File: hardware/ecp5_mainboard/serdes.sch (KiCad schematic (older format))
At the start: 48 parts, among them J14 9774025151R, J8 9774025151R, P1 M2_SOCKET_E, P3 PCIe_x4_EDGE, U11 CBTL02043A, U15 ECP5UM5G_85_CABGA756, U16 5P49V6965, Y1 25MHz

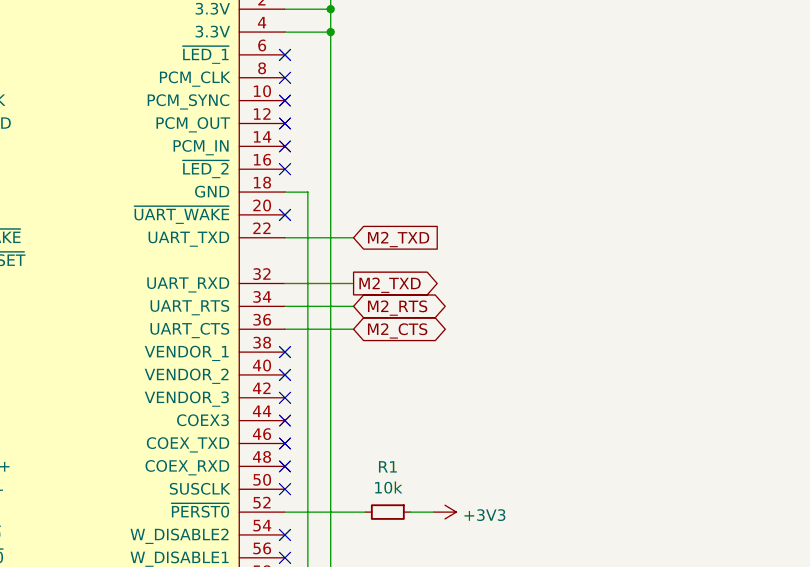
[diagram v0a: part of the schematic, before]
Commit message: hardware/mainboard: Clock & M.2 routing
Signed-off-by: David Shah <davey1576@gmail.com>
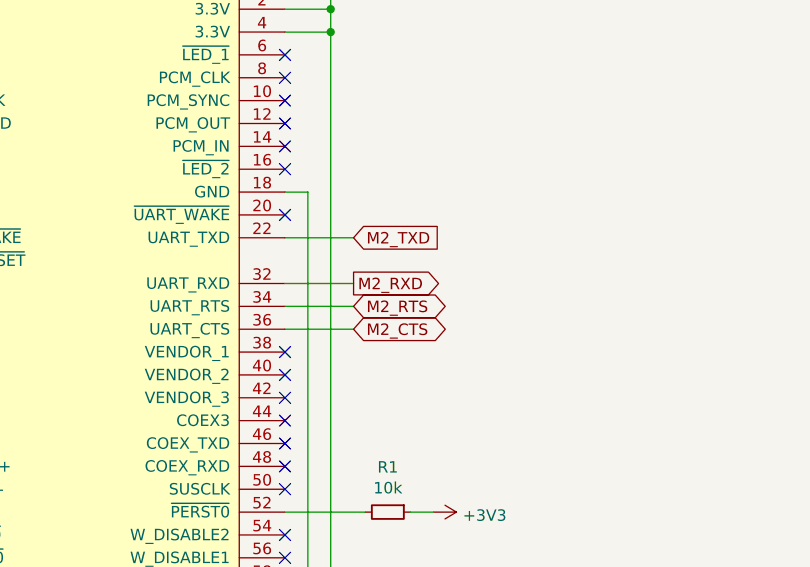
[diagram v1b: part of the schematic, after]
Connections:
- net M2_TXD: no longer P1.32 (UART_RXD)
- new net M2_RXD: P1.32 (UART_RXD)
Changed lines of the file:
@@
 M2_TXD
 Text GLabel 9200 7500 2    50   Output ~ 0
-M2_TXD
+M2_RXD
 Wire Wire Line
 	9200 7500 8900 7500
